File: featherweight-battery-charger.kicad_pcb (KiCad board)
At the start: 2 copper layers, 16 parts, among them J1 G125-MH104M4-04AD000P, J2 Conn_01x02, U1 MCP73832-2-OT, U2 TPS561208DDCR

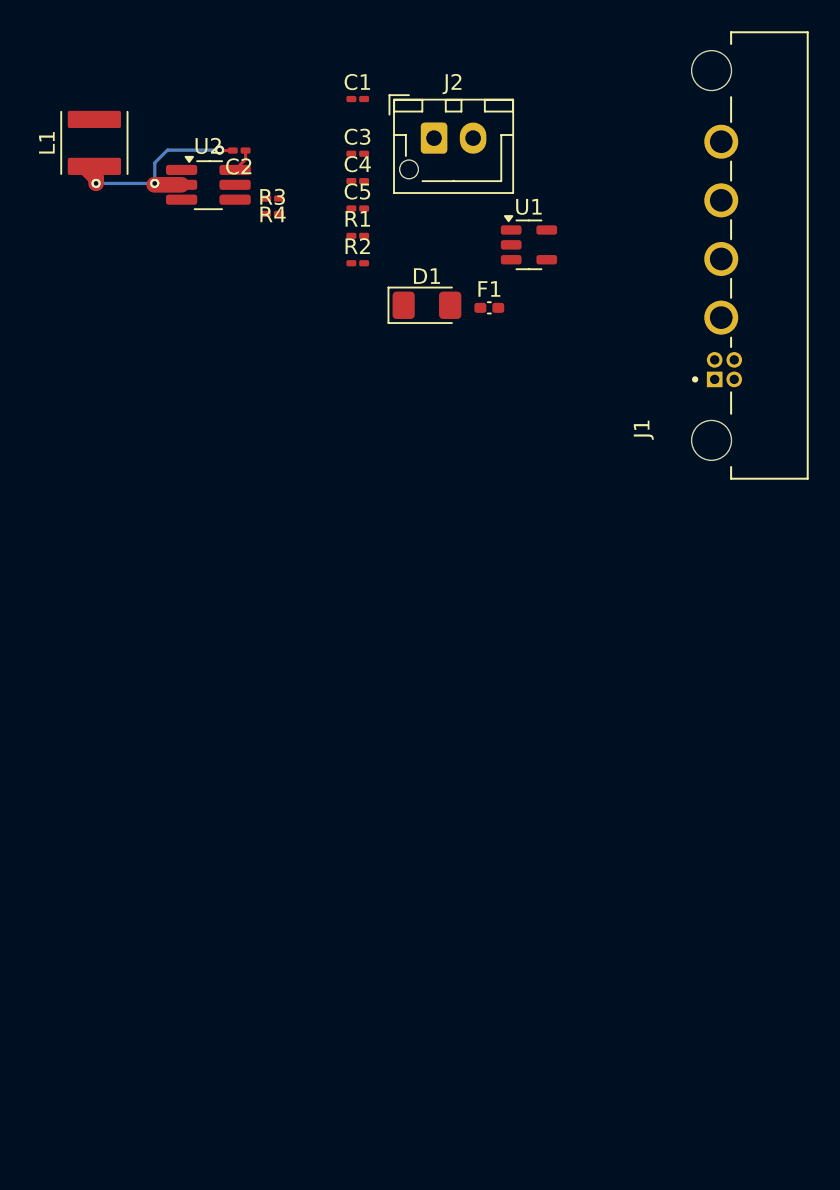
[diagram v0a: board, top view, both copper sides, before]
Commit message: Started Layout and Routing
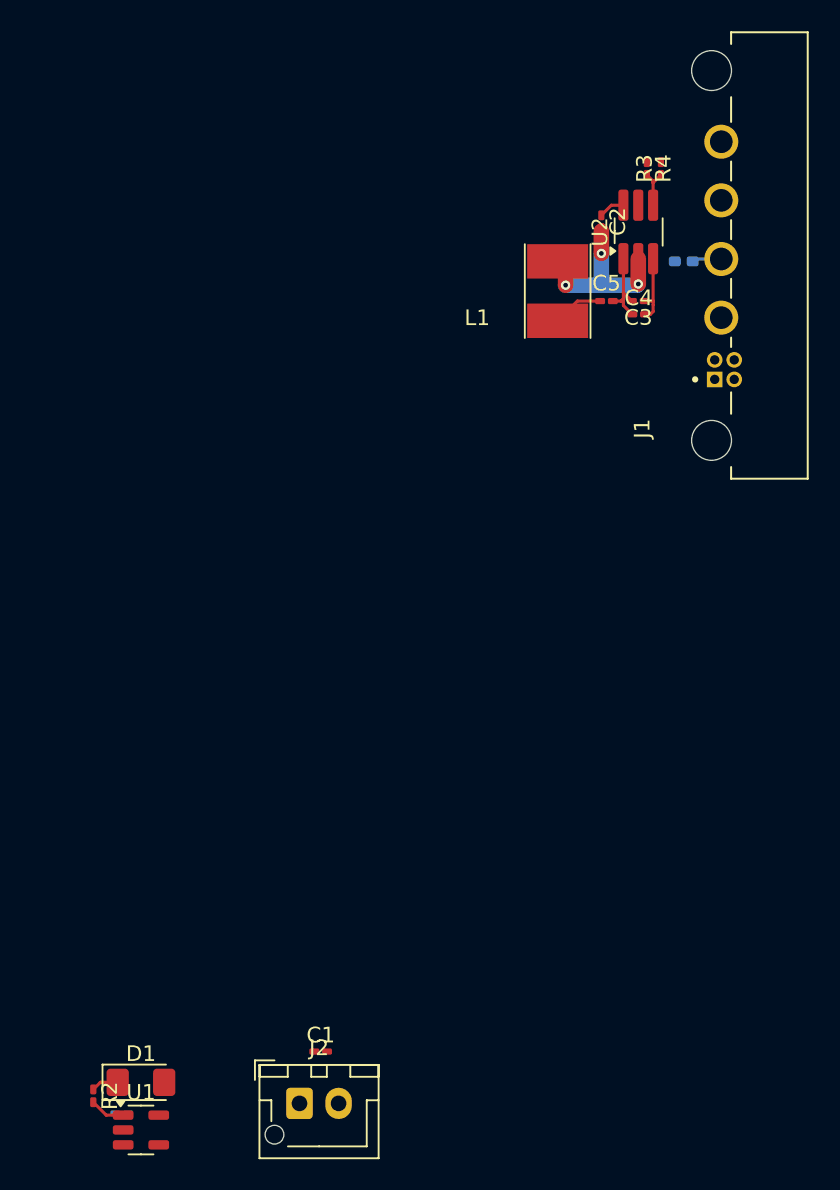
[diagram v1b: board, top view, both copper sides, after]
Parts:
- F1, R1: moved to B.Cu
- L1: value ASPI-4030S-4R7M-T (4.7uH) -> NRS4018T4R7MDGJ (4.7uH); footprint Inductor_SMD:L_Abracon_ASPI-4030S -> Inductor_SMD:L_Taiyo-Yuden_NR-40xx_HandSoldering
- moved J2 62.3 mm to (125.0, 119.6)
- moved U1 61.8 mm to (114.8, 121.3)
- moved C1 61.0 mm to (126.3, 116.3)
- moved R1 58.1 mm to (113.6, 120.3), turned to 180 degrees
- moved R2 55.9 mm to (111.8, 119.1), turned to -90 degrees
- moved D1 53.0 mm to (114.8, 118.3)
- moved L1 31.1 mm to (141.5, 67.7), turned to -90 degrees
- moved U2 27.7 mm to (146.6, 63.9), turned to 90 degrees
- moved R3 25.0 mm to (148.1, 59.8), turned to 90 degrees
- moved R4 24.0 mm to (147.2, 59.8), turned to -90 degrees
- moved C2 23.6 mm to (144.3, 63.2), turned to -90 degrees
- moved C3 20.3 mm to (146.6, 68.3), turned to 180 degrees
- moved C4 19.9 mm to (146.7, 69.2)
- moved C5 17.0 mm to (144.6, 68.3), turned to 180 degrees
- moved F1 12.8 mm to (149.5, 65.8), turned to 180 degrees
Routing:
- net GND: track 0.00 -> 5.30 mm
- net +12V: track 0.00 -> 4.77 mm
- net +5V: track 0.00 -> 3.24 mm
- net Net-(U2-VFB): track 0.00 -> 2.81 mm
- net Net-(U2-SW): track 13.8 -> 11.5 mm
- net /STAT: track 0.00 -> 2.25 mm
- net Net-(J1-+12V): track 0.00 -> 1.89 mm
- net Net-(D1-K): track 0.00 -> 1.75 mm
